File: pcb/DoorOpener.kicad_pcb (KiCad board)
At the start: 2 copper layers, 48 x 37.7 mm, 8 parts, among them J1 Serial, SW1 POWER, SW2 Button, U2 ESP-01v090

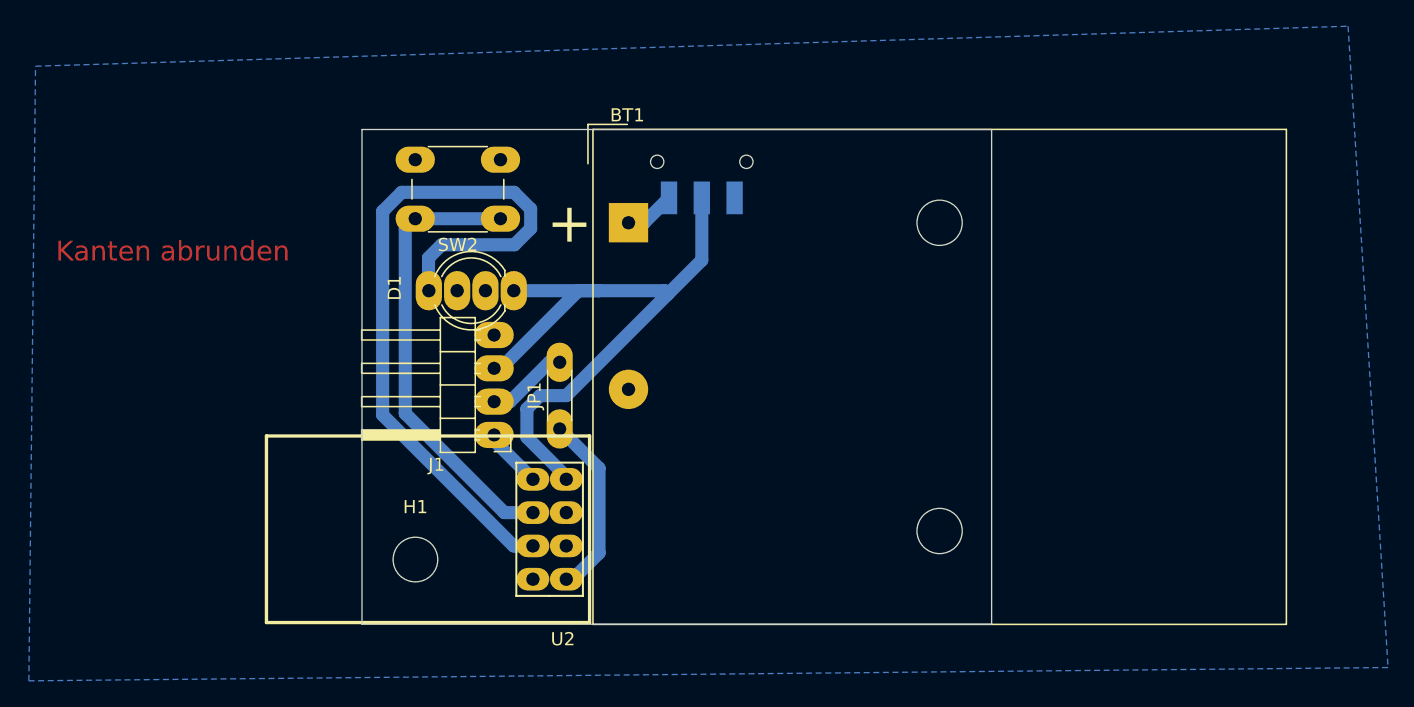
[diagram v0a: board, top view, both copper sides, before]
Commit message: Version 0.2
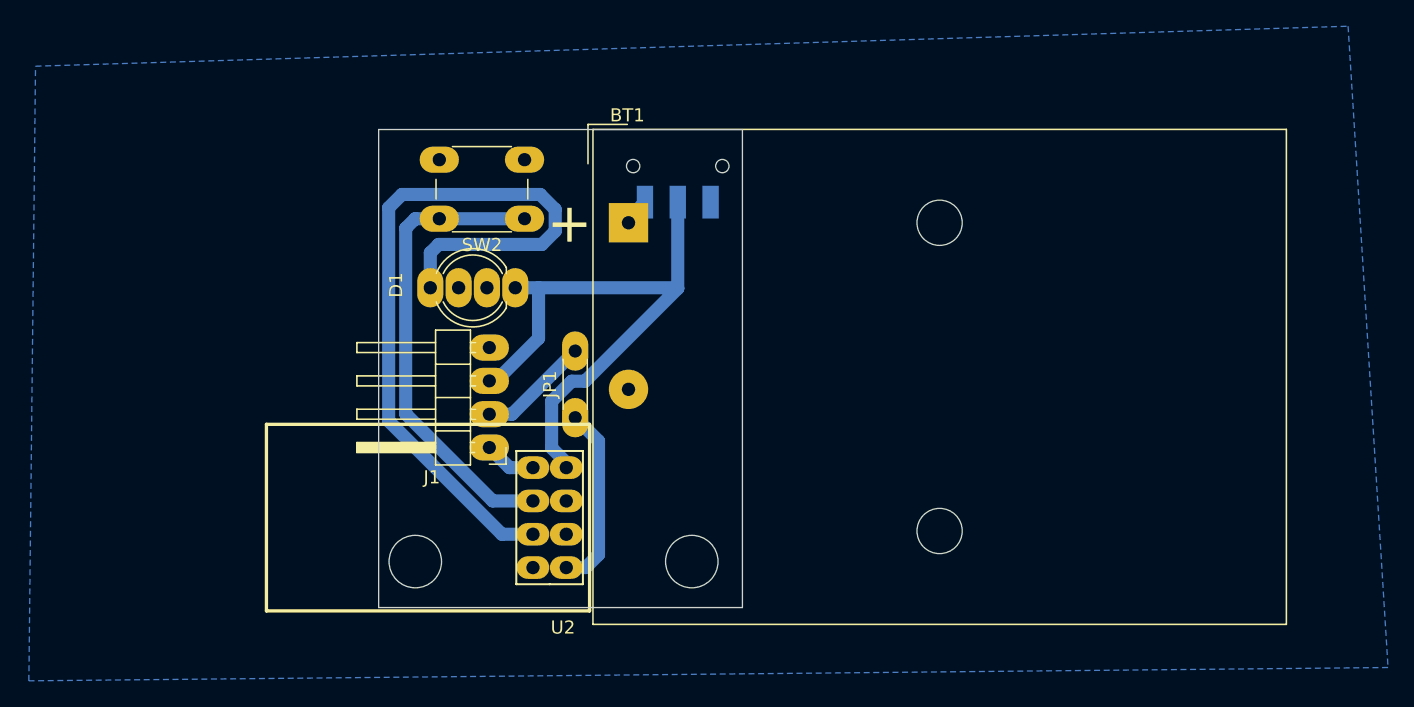
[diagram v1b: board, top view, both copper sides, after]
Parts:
- removed H1: MountingHole, MountingHole:MountingHole_3mm
- moved SW1 1.86 mm to (96.2, 125.3)
- moved SW2 1.83 mm to (84.5, 129.4)
- moved JP1 1.46 mm to (88.4, 144.5)
- moved J1 1.02 mm to (81.8, 146.8)
- moved U2 0.89 mm to (87.7, 156.0)
- moved D1 0.25 mm to (83.8, 134.6)
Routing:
- net +3V3: track 51.7 -> 46.6 mm
- net Net-(D1-Pad4): track 55.7 -> 59.0 mm
- net Net-(J1-Pad2): track 6.13 -> 8.54 mm
- net Net-(BT1-Pad1): track 3.87 -> 2.09 mm
- net Net-(SW2-Pad1): track 34.5 -> 36.0 mm
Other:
- board size 48 x 37.7 mm -> 27.7 x 36.4 mm
- board text added: "v0.2 - 3.12.2022"
- board text removed: "Kanten abrunden"
- board text removed: "v0.1 - 17.11.2022"
